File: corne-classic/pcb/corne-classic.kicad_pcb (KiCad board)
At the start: 2 copper layers, 133.8 x 92.2 mm, 98 parts, among them J1 MJ-4PP-9, J2 OLED, J3 LED, P1 i2c-pin, P2 i2c-pin, SW1 SW_PUSH, SW10 SW_PUSH, SW11 SW_PUSH, SW12 SW_PUSH, SW13 SW_PUSH, SW14 SW_PUSH, SW15 SW_PUSH, SW16 SW_PUSH, SW17 SW_PUSH, SW18 SW_PUSH, SW19 SW_PUSH, SW2 SW_PUSH, SW20 SW_PUSH, SW21 SW_PUSH, SW3 SW_PUSH, SW4 SW_PUSH, SW5 SW_PUSH, SW6 SW_PUSH, SW7 SW_PUSH, SW8 SW_PUSH, SW9 SW_PUSH, U1 ProMicro

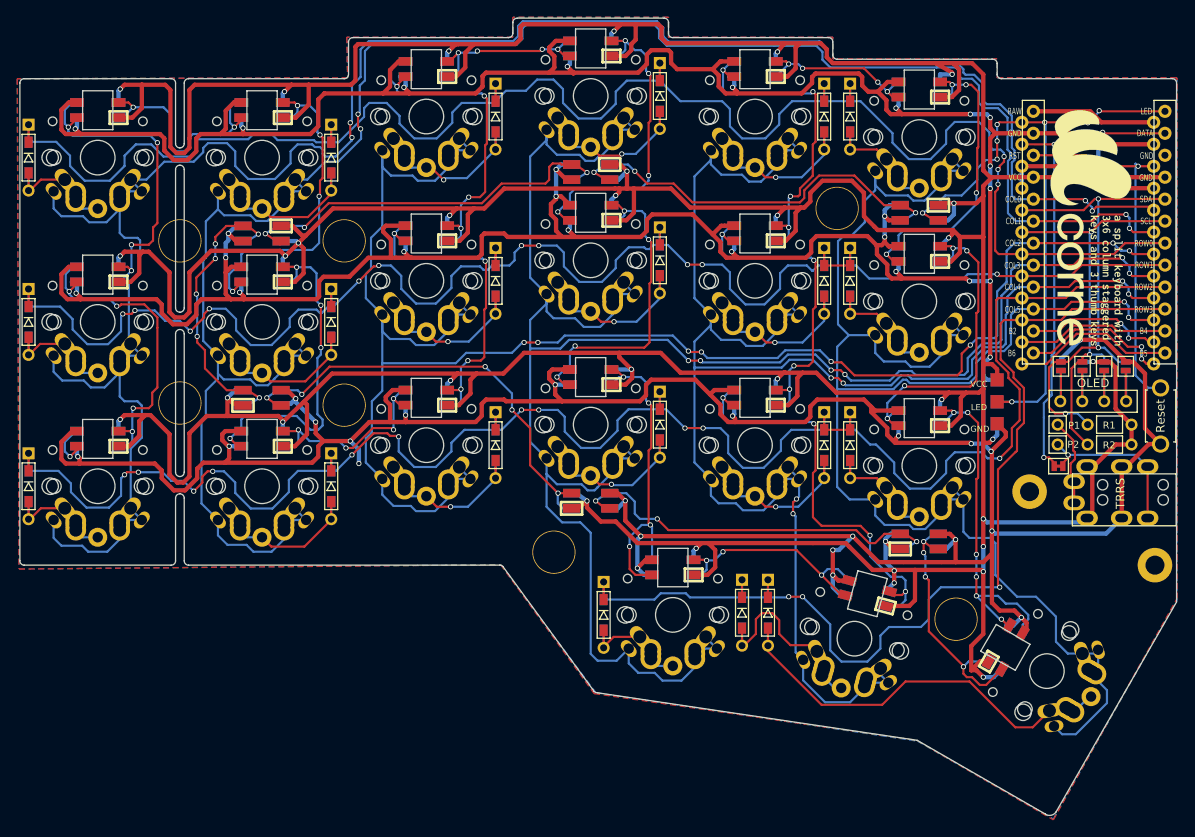
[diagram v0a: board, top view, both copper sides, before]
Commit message: new footprint for Choc V2 switches
added new footprints, tracks need work
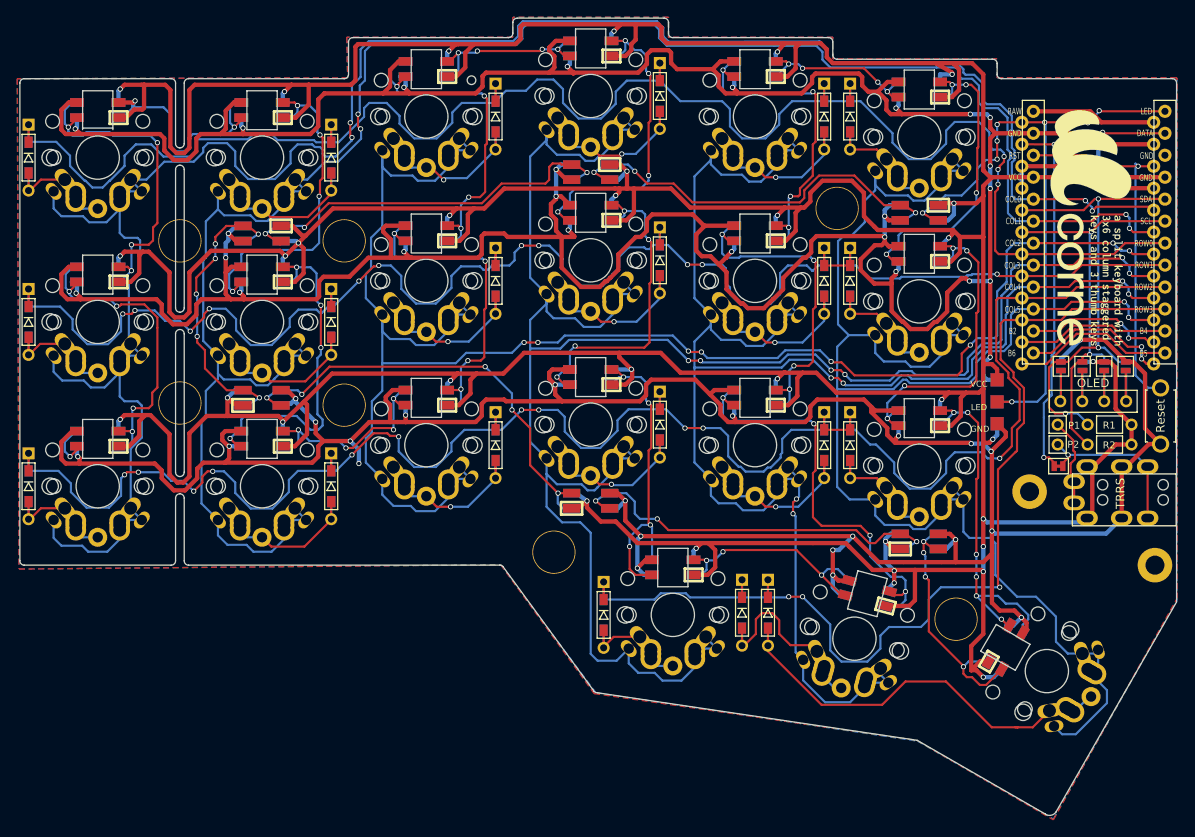
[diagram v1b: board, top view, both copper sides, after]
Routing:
- net GND: track 797.7 -> 830.1 mm
- net Net-(L1-Pad1): track 37.7 -> 40.6 mm
- net Net-(L1-Pad3): track 27.6 -> 29.6 mm
- net row1: track 191.7 -> 193.1 mm
- net row2: track 215.8 -> 216.8 mm
- net row0: track 205.5 -> 206.2 mm
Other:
- outline, holes or cut-outs redrawn
